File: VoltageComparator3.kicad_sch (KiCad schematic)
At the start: 6 parts, among them U18 LM324, U19 74LS08

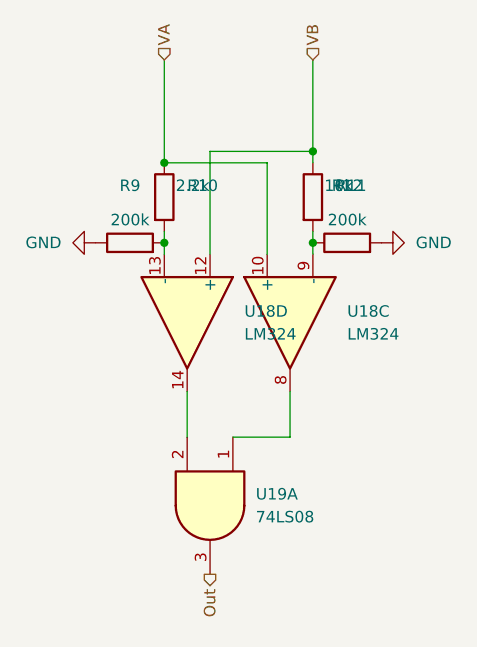
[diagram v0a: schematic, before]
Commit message: Ground and Power Plane?
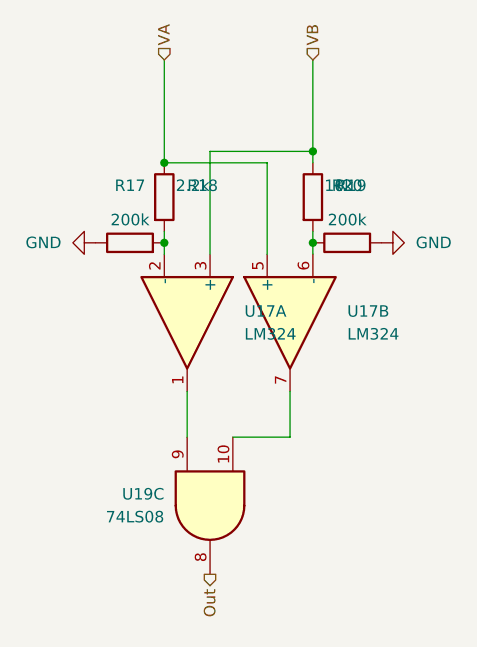
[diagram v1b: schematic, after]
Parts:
- renumbered R9 to R17, R10 to R18, R11 to R19, R12 to R20, U18 to U17
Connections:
- net Out: now also U19.8; no longer U19.3
- net VA: now also U17.5 (+); no longer U17.10 (+)
- net VB: now also U17.3 (+); no longer U17.12 (+)
- net at R17.2, R18.2: now also U17.2 (-); no longer U17.13 (-)
- net at R19.2, R20.1: now also U17.6 (-); no longer U17.9 (-)
- new net: U17.7, U19.10
- new net: U17.1, U19.9
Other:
- moved on the sheet: U19C
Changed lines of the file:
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@@
 	(symbol
 		(lib_id "74xx:74LS08")
-		(at 53.34 96.52 270)
-		(unit 1)
+		(at 53.34 96.52 90)
+		(mirror x)
+		(unit 3)
 		(exclude_from_sim no)
 		(in_bom yes)
@@
 		(dnp no)
 		(property "Reference" "U19"
-			(at 58.42 95.2416 90)
+			(at 48.26 95.2416 90)
 			(effects
 				(font
@@
 		)
 		(property "Value" "74LS08"
-			(at 58.42 97.7816 90)
+			(at 48.26 97.7816 90)
 			(effects
 				(font
@@
 		)
 		(instances
-			(project ""
+			(project "ECE145Mastermind"
 				(path "/8c64fe8a-5d6b-41bc-b3a3-9bda7b2e0f2c/218d925b-79f6-474b-97b2-c0ad78559cda"
 					(reference "U19")
 					(unit 3)
-				)
-				(path "/8c64fe8a-5d6b-41bc-b3a3-9bda7b2e0f2c/4f59e726-7fd4-4ef0-8dbb-7a41976aa953"
-					(reference "U19")
-					(unit 1)
-				)
-				(path "/8c64fe8a-5d6b-41bc-b3a3-9bda7b2e0f2c/acb554fe-df67-46ea-bc1c-079edbbfc216"
-					(reference "U19")
-					(unit 2)
-				)
-				(path "/8c64fe8a-5d6b-41bc-b3a3-9bda7b2e0f2c/d4674d5d-47f2-4c8d-9fae-4e866cda3652"
-					(reference "U19")
-					(unit 4)
 				)
 			)
@@
 		(dnp no)
 		(fields_autoplaced yes)
-		(property "Reference" "#PWR088"
+		(property "Reference" "#PWR092"
 			(at 78.74 67.31 0)
 			(effects
@@
 		(instances
 			(project "ECE145Mastermind"
-				(path "/8c64fe8a-5d6b-41bc-b3a3-9bda7b2e0f2c/4f59e726-7fd4-4ef0-8dbb-7a41976aa953"
-					(reference "#PWR088")
+				(path "/8c64fe8a-5d6b-41bc-b3a3-9bda7b2e0f2c/218d925b-79f6-474b-97b2-c0ad78559cda"
+					(reference "#PWR092")
 					(unit 1)
 				)
@@
 		(on_board yes)
 		(dnp no)
-		(property "Reference" "R10"
+		(property "Reference" "R18"
 			(at 50.8 60.9599 0)
 			(effects
@@
 		(instances
 			(project "ECE145Mastermind"
-				(path "/8c64fe8a-5d6b-41bc-b3a3-9bda7b2e0f2c/4f59e726-7fd4-4ef0-8dbb-7a41976aa953"
-					(reference "R10")
+				(path "/8c64fe8a-5d6b-41bc-b3a3-9bda7b2e0f2c/218d925b-79f6-474b-97b2-c0ad78559cda"
+					(reference "R18")
 					(unit 1)
 				)
@@
 		(dnp no)
 		(fields_autoplaced yes)
-		(property "Reference" "#PWR087"
+		(property "Reference" "#PWR091"
 			(at 34.29 67.31 0)
 			(effects
@@
 		(instances
 			(project "ECE145Mastermind"
-				(path "/8c64fe8a-5d6b-41bc-b3a3-9bda7b2e0f2c/4f59e726-7fd4-4ef0-8dbb-7a41976aa953"
-					(reference "#PWR087")
+				(path "/8c64fe8a-5d6b-41bc-b3a3-9bda7b2e0f2c/218d925b-79f6-474b-97b2-c0ad78559cda"
+					(reference "#PWR091")
 					(unit 1)
 				)
@@
 		(on_board yes)
 		(dnp no)
-		(property "Reference" "R11"
+		(property "Reference" "R19"
 			(at 67.31 60.9599 0)
 			(effects
@@
 		(instances
 			(project "ECE145Mastermind"
-				(path "/8c64fe8a-5d6b-41bc-b3a3-9bda7b2e0f2c/4f59e726-7fd4-4ef0-8dbb-7a41976aa953"
-					(reference "R11")
+				(path "/8c64fe8a-5d6b-41bc-b3a3-9bda7b2e0f2c/218d925b-79f6-474b-97b2-c0ad78559cda"
+					(reference "R19")
 					(unit 1)
 				)
@@
 		(at 62.23 76.2 90)
 		(mirror x)
-		(unit 3)
+		(unit 2)
 		(exclude_from_sim no)
 		(in_bom yes)
@@
 		(dnp no)
 		(fields_autoplaced yes)
-		(property "Reference" "U18"
+		(property "Reference" "U17"
 			(at 68.58 74.9299 90)
 			(effects
@@
 		(instances
 			(project "ECE145Mastermind"
-				(path "/8c64fe8a-5d6b-41bc-b3a3-9bda7b2e0f2c/4f59e726-7fd4-4ef0-8dbb-7a41976aa953"
-					(reference "U18")
-					(unit 3)
+				(path "/8c64fe8a-5d6b-41bc-b3a3-9bda7b2e0f2c/218d925b-79f6-474b-97b2-c0ad78559cda"
+					(reference "U17")
+					(unit 2)
 				)
 			)
@@
 		(lib_id "Amplifier_Operational:LM324")
 		(at 50.8 76.2 270)
-		(unit 4)
+		(unit 1)
 		(exclude_from_sim no)
 		(in_bom yes)
@@
 		(dnp no)
 		(fields_autoplaced yes)
-		(property "Reference" "U18"
+		(property "Reference" "U17"
 			(at 57.15 74.9299 90)
 			(effects
@@
 		(instances
 			(project "ECE145Mastermind"
-				(path "/8c64fe8a-5d6b-41bc-b3a3-9bda7b2e0f2c/4f59e726-7fd4-4ef0-8dbb-7a41976aa953"
-					(reference "U18")
-					(unit 4)
+				(path "/8c64fe8a-5d6b-41bc-b3a3-9bda7b2e0f2c/218d925b-79f6-474b-97b2-c0ad78559cda"
+					(reference "U17")
+					(unit 1)
 				)
 			)
@@
 		(on_board yes)
 		(dnp no)
-		(property "Reference" "R9"
+		(property "Reference" "R17"
 			(at 44.45 60.96 90)
 			(effects
@@
 		(instances
 			(project "ECE145Mastermind"
-				(path "/8c64fe8a-5d6b-41bc-b3a3-9bda7b2e0f2c/4f59e726-7fd4-4ef0-8dbb-7a41976aa953"
-					(reference "R9")
+				(path "/8c64fe8a-5d6b-41bc-b3a3-9bda7b2e0f2c/218d925b-79f6-474b-97b2-c0ad78559cda"
+					(reference "R17")
 					(unit 1)
 				)
@@
 		(on_board yes)
 		(dnp no)
-		(property "Reference" "R12"
+		(property "Reference" "R20"
 			(at 68.58 60.96 90)
 			(effects
@@
 		(instances
 			(project "ECE145Mastermind"
-				(path "/8c64fe8a-5d6b-41bc-b3a3-9bda7b2e0f2c/4f59e726-7fd4-4ef0-8dbb-7a41976aa953"
-					(reference "R12")
+				(path "/8c64fe8a-5d6b-41bc-b3a3-9bda7b2e0f2c/218d925b-79f6-474b-97b2-c0ad78559cda"
+					(reference "R20")
 					(unit 1)
 				)

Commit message: Finished?
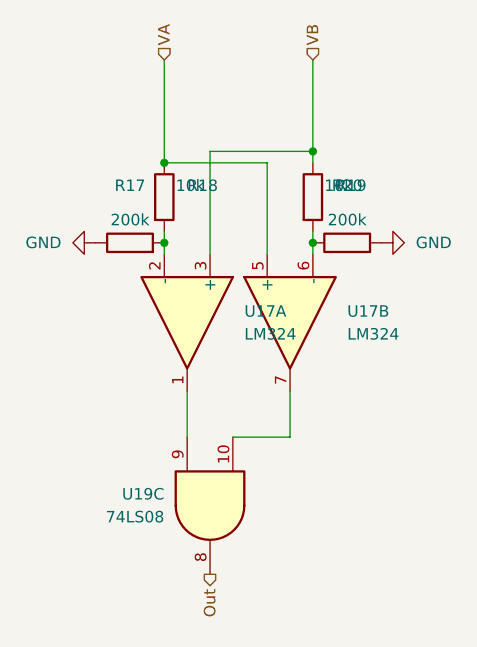
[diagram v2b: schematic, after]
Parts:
- R18: value 2.2k -> 10k
